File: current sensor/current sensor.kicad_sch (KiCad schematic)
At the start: 25 parts, among them U1 ACS711xLCTR-25AB, U2 ACS711xLCTR-25AB, U3 ACS711xLCTR-25AB, U4 ACS711xLCTR-25AB, U4 ADS7830, U5 ACS711xLCTR-25AB, U6 ACS711xLCTR-25AB

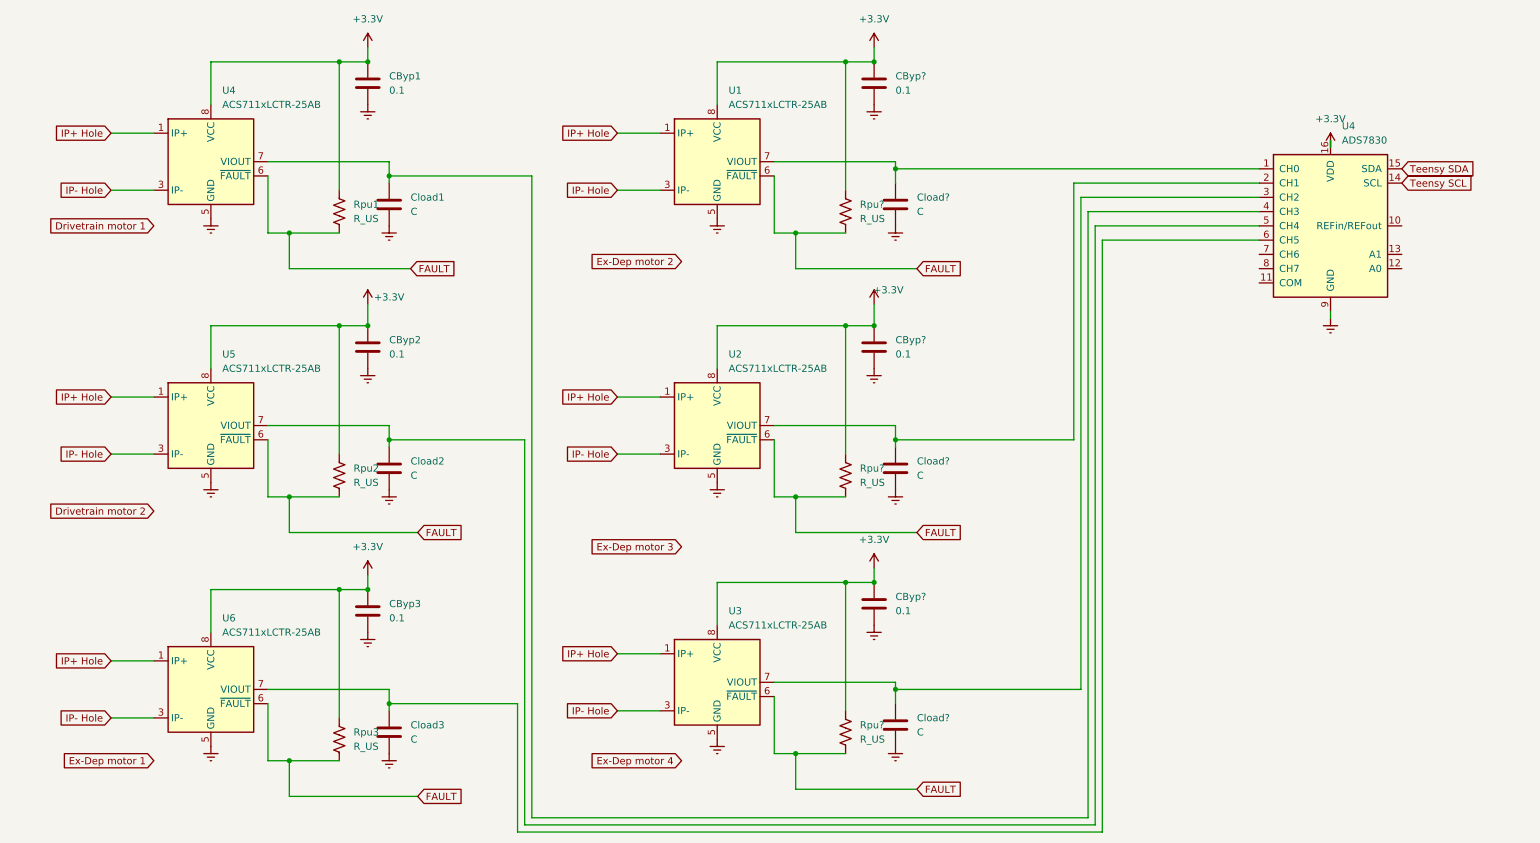
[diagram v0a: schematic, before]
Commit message: Add files via upload
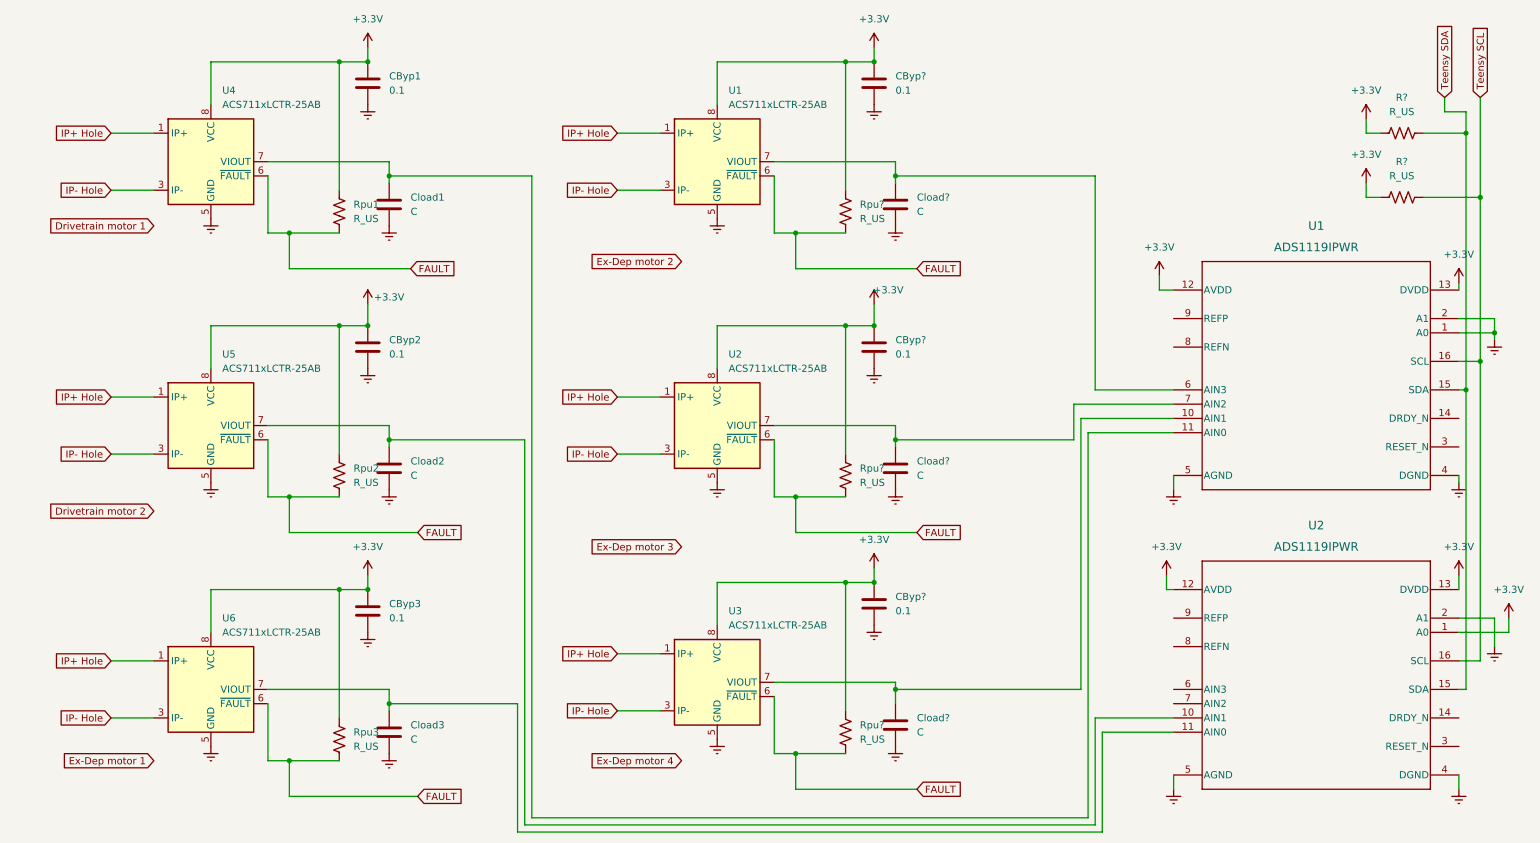
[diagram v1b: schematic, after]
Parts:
- removed U4: ADS7830, Package_SO:TSSOP-16_4.4x5mm_P0.65mm, symbol Analog_DAC:ADS7830
- added R? (x2): R_US, symbol Device:R_US
- added U1, U2: ADS1119IPWR, PW0016A_N, symbol 2023-10-21_17-11-10:ADS1119IPWR
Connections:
- net +3.3V: now also R?.1, R?.1, U1.12 (AVDD), U1.13 (DVDD), U2.1 (A0), U2.12 (AVDD), U2.13 (DVDD)
- net Earth: now also U1.1 (A0), U1.2 (A1), U1.4 (DGND), U1.5 (AGND), U2.2 (A1), U2.4 (DGND), U2.5 (AGND)
- net Teensy SCL: now also R?.2, U1.16 (SCL), U2.16 (SCL)
- net Teensy SDA: now also R?.2, U1.15 (SDA), U2.15 (SDA)
- net at Cload2.1, U5.7 (VIOUT): now also U2.10 (AIN1)
- net at Cload3.1, U6.7 (VIOUT): now also U2.11 (AIN0)
- net at Cload?.1, U2.7 (VIOUT): now also U1.7 (AIN2)
- net at Cload1.1, U4.7 (VIOUT): now also U1.11 (AIN0)
- net at Cload?.1, U3.7 (VIOUT): now also U1.10 (AIN1)
- net at Cload?.1, U1.7 (VIOUT): now also U1.6 (AIN3)
